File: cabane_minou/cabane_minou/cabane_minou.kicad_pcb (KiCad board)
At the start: 2 copper layers, 176 x 120 mm, 135 parts, among them J1 Alim 12V, J10 Serial, J11 LEDs Res, J12 Leds, J13 Buttons, J14 Couvercle, J15 Commande 12V, J2 Log, J3 Screen, J4 Bas, J5 LEDs Bas, J6 Move Tour, J7 LEDs Tour, J8 Move Haut, J9 LEDs Haut, Q1 BPC_2N2222A, Q10 BC327, Q11 BPC_2N2222A, Q12 BPC_2N2222A, Q13 BC327, Q14 BC327, Q2 BC327, Q3 BPC_2N2222A, Q4 BC327, Q5 BPC_2N2222A, Q6 BPC_IPP034N03L, Q7 BPC_2N2222A, Q8 BPC_2N2222A, Q9 BC327, U1 BPC_Alim5V, U2 LM1117DT-3.3, U3 BPC_ATMEGA2560_PRO, U5 RtcArduino, U6 BPC_ESP8266-01_ESP-01, X1 Trou, X2 Trou, X3 Trou, X4 Trou

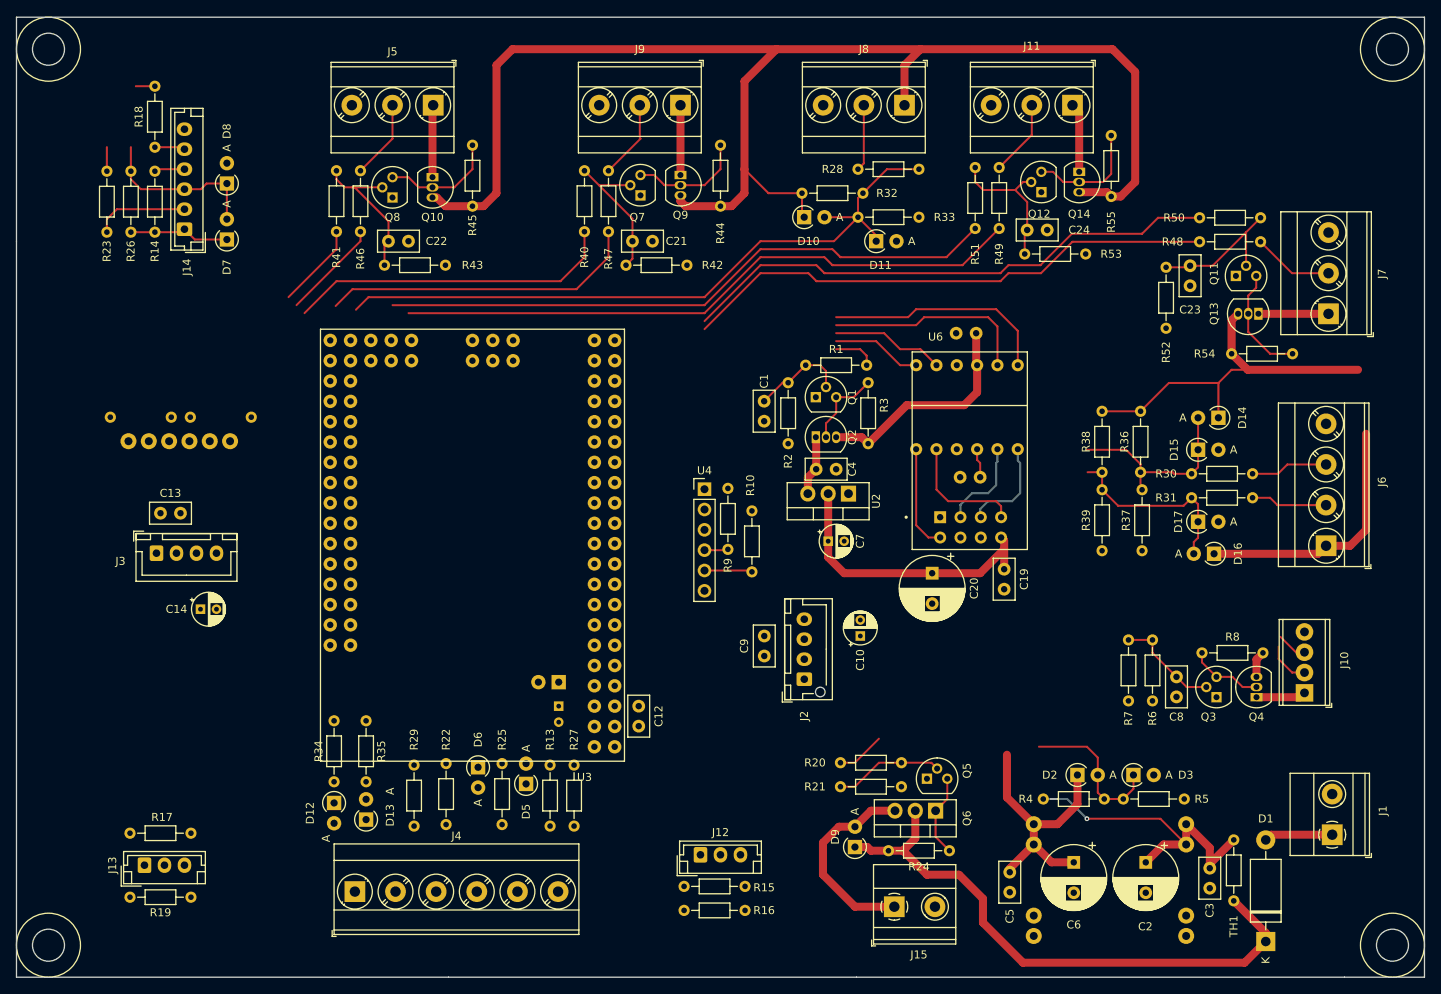
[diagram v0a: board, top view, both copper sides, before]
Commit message: Design cabane minou "version 2024"
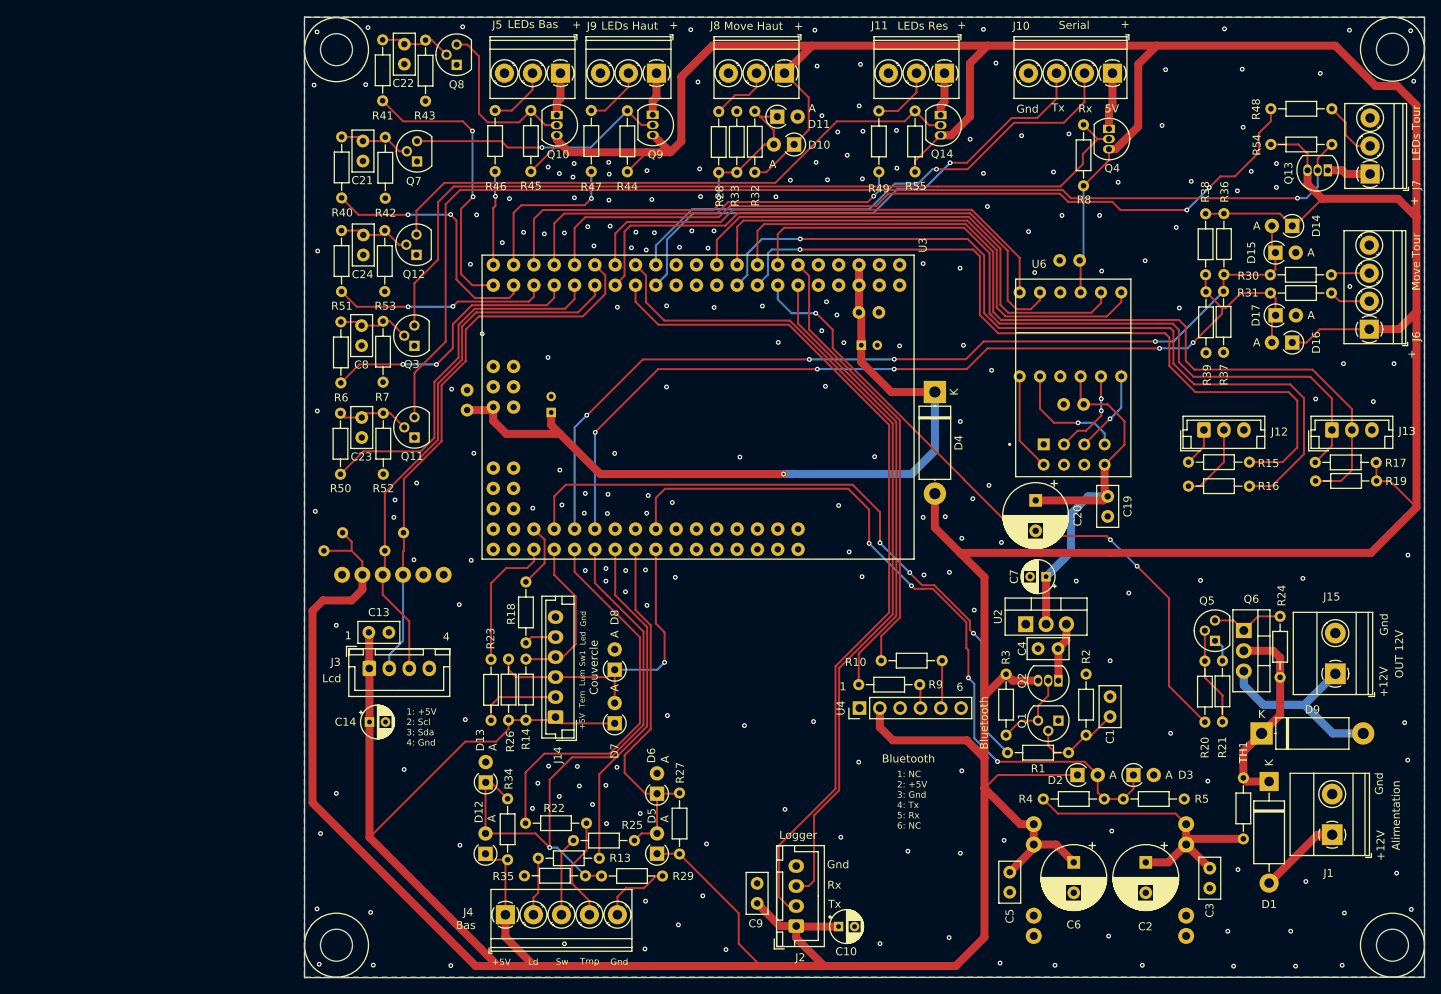
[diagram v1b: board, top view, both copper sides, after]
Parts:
- added C15: 10uF, Capacitor_THT:CP_Radial_D4.0mm_P2.00mm, B.Cu at (104.8, 72.4)
- added C17: 1n, Capacitor_THT:C_Disc_D5.0mm_W2.5mm_P2.50mm, B.Cu at (94.3, 72.1)
- C12: moved to B.Cu
- D4: footprint Diode_THT:D_A-405_P2.54mm_Vertical_AnodeUp -> Diode_THT:D_5W_P12.70mm_Horizontal; moved to F.Cu
- D9: footprint Diode_THT:D_A-405_P2.54mm_Vertical_AnodeUp -> Diode_THT:D_5W_P12.70mm_Horizontal
- J10: footprint TerminalBlock_Phoenix:TerminalBlock_Phoenix_MPT-0,5-4-2.54_1x04_P2.54mm_Horizontal -> TerminalBlock_Phoenix:TerminalBlock_Phoenix_PT-1,5-4-3.5-H_1x04_P3.50mm_Horizontal
- J11, J5, J7, J8, J9: footprint TerminalBlock_Phoenix:TerminalBlock_Phoenix_MKDS-3-3-5.08_1x03_P5.08mm_Horizontal -> TerminalBlock_Phoenix:TerminalBlock_Phoenix_PT-1,5-3-3.5-H_1x03_P3.50mm_Horizontal
- J2: footprint Connector_JST:JST_XH_B4B-XH-AM_1x04_P2.50mm_Vertical -> Connector_JST:JST_XH_B4B-XH-A_1x04_P2.50mm_Vertical
- J4: footprint TerminalBlock_Phoenix:TerminalBlock_Phoenix_MKDS-3-6-5.08_1x06_P5.08mm_Horizontal -> TerminalBlock_Phoenix:TerminalBlock_Phoenix_PT-1,5-5-3.5-H_1x05_P3.50mm_Horizontal
- J6: footprint TerminalBlock_Phoenix:TerminalBlock_Phoenix_MKDS-3-4-5.08_1x04_P5.08mm_Horizontal -> TerminalBlock_Phoenix:TerminalBlock_Phoenix_PT-1,5-4-3.5-H_1x04_P3.50mm_Horizontal
- moved J13 158.1 mm to (202.4, 74.6)
- moved R19 157.1 mm to (208.0, 81.0)
- moved R17 155.2 mm to (208.0, 78.7)
- moved R50 112.1 mm to (78.5, 80.1), turned to 90 degrees
- moved C8 110.9 mm to (81.1, 61.5)
- moved Q3 109.5 mm to (87.7, 64.1)
- moved R6 109.0 mm to (78.5, 68.7)
- moved C23 105.3 mm to (81.2, 73.0)
- moved Q11 104.6 mm to (87.8, 75.5), turned to 90 degrees
- moved R7 101.3 mm to (83.8, 61.0)
- moved R52 99.5 mm to (83.8, 72.5)
- moved C24 83.0 mm to (81.3, 50.2), turned to -90 degrees
- moved R15 82.4 mm to (184.5, 78.6)
- moved R16 82.4 mm to (184.5, 81.6)
- moved J12 82.3 mm to (186.4, 74.6)
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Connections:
- U3 pad A0: UC_IN_MES_12V -> unconnected-(U3-PadA0)
- U3 pad A1: LUMINOSITE -> unconnected-(U3-PadA1)
- U3 pad A14: unconnected-(U3-PadA14) -> LUMINOSITE
- U3 pad A15: unconnected-(U3-PadA15) -> UC_IN_MES_12V
- U3 pad D2: UC_OUT_LED_1 -> UC_OUT_CMD_CHAUFFAGE
- U3 pad D22: UC_IO1 -> UC_5V_LEDS_TOUR
- U3 pad D23: UC_5V_LEDS_TOUR -> UC_OUT_LEDS_TOUR
- U3 pad D24: UC_IO2 -> UC_5V_SER
- U3 pad D26: UC_5V_LEDS_BAS -> UC_5V_LEDS_RES
- U3 pad D27: UC_5V_LEDS_RES -> UC_IN_PRESENCE_HAUT
- U3 pad D28: UC_OUT_LEDS_BAS -> UC_5V_LEDS_HAUT
- U3 pad D29: UC_IN_PRESENCE_HAUT -> UC_OUT_LEDS_HAUT
- U3 pad D3: UC_IN_SW1_BUTTON -> UC_IN_SW2_BUTTON
- U3 pad D30: UC_5V_LEDS_HAUT -> UC_5V_LEDS_BAS
- U3 pad D31: UC_OUT_LEDS_HAUT -> UC_OUT_LEDS_BAS
- U3 pad D32: unconnected-(U3-PadD32) -> UC_IN_CAPOT
- U3 pad D34: unconnected-(U3-PadD34) -> UC_OUT_LED_CAPOT_OUVERT
- U3 pad D35: UC_5V_SER -> unconnected-(U3-PadD35)
- U3 pad D36: unconnected-(U3-PadD36) -> UC_IN_PRESENCE_BAS
- U3 pad D37: unconnected-(U3-PadD37) -> UC_IN_PRESENCE_TOUR_BAS
- U3 pad D38: UC_IN_PRESENCE_BAS -> UC_TEMP_BAS
- U3 pad D39: unconnected-(U3-PadD39) -> UC_IN_PRESENCE_TOUR_HAUT
- U3 pad D40: UC_OUT_LED_CAPOT_OUVERT -> UC_IN_SW1_BUTTON
- U3 pad D41: UC_IN_CAPOT -> UC_3V_ESP
- U3 pad D43: UC_TEMP_BAS -> UC_OUT_LED_1
- U3 pad D45: UC_OUT_CMD_CHAUFFAGE -> unconnected-(U3-PadD45)
- U3 pad D5: UC_IN_SW2_BUTTON -> UC_IN_SW3_BUTTON
- U3 pad D7: UC_IN_SW3_BUTTON -> UC_IO1
- U3 pad D9: UC_3V_ESP -> UC_IO2
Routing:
- net +5V: track 333.7 -> 785.2 mm
- net Net-(Q13-B): track 14.1 -> 145.0 mm, vias 0 -> 1
- net UC_IN_SW3_BUTTON: track 0.00 -> 108.1 mm
- net UC_TX_LOG: track 0.00 -> 107.5 mm
- net UC_RX_LOG: track 0.00 -> 106.1 mm
- net UC_OUT_LED_3: track 0.00 -> 105.1 mm, vias 0 -> 1
- net UC_IN_SW2_BUTTON: track 0.00 -> 97.9 mm
- net Net-(D4-K): track 0.00 -> 97.8 mm, vias 0 -> 1
- net Net-(Q4-B): track 9.28 -> 107.0 mm
- net UC_OUT_LED_2: track 0.00 -> 97.7 mm, vias 0 -> 1
- net UC_IN_PRESENCE_TOUR_BAS: track 24.0 -> 115.8 mm, vias 0 -> 5
- net UC_IN_PRESENCE_TOUR_HAUT: track 24.6 -> 115.4 mm, vias 0 -> 4
- net UC_OUT_CMD_CHAUFFAGE: track 6.05 -> 85.9 mm, vias 0 -> 3
- net UC_3V_ESP: track 5.34 -> 84.4 mm, vias 0 -> 3
- net UC_IN_MES_12V: track 19.3 -> 94.1 mm, vias 0 -> 4
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- added copper zone on B.Cu, net GND
- added copper zone on F.Cu, net GND
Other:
- board size 176 x 120 mm -> 140 x 120.1 mm
- board text added: "+"
- board text added: "+12V"
- board text added: "+5V"
- board text added: "1"
- board text added: "1: +5V 2: Scl 3: Sda 4: Gnd"
- board text added: "1: NC 2: +5V 3: Gnd 4: Tx 5: Rx 6: NC"
- board text added: "4"
- board text added: "5V"
- board text added: "6"
- board text added: "Alimentation"
- board text added: "Bas"
- board text added: "Bluetooth"
- board text added: "Couvercle"
- board text added: "Gnd"
- board text added: "LEDs Bas"
- board text added: "LEDs Haut"
- board text added: "LEDs Res"
- board text added: "LEDs Tour"
- board text added: "Lcd"
- board text added: "Ld"
- board text added: "Led"
- board text added: "Logger"
- board text added: "Lum"
- board text added: "Move Haut"
- board text added: "Move Tour"
- board text added: "OUT 12V"
- board text added: "Rx"
- board text added: "Serial"
- board text added: "Sw"
- board text added: "Sw1"
- board text added: "Tem"
- board text added: "Tmp"
- board text added: "Tx"
